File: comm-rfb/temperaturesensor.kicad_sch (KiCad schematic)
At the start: 5 parts, among them U4 MCP9808T-E{slash}MC

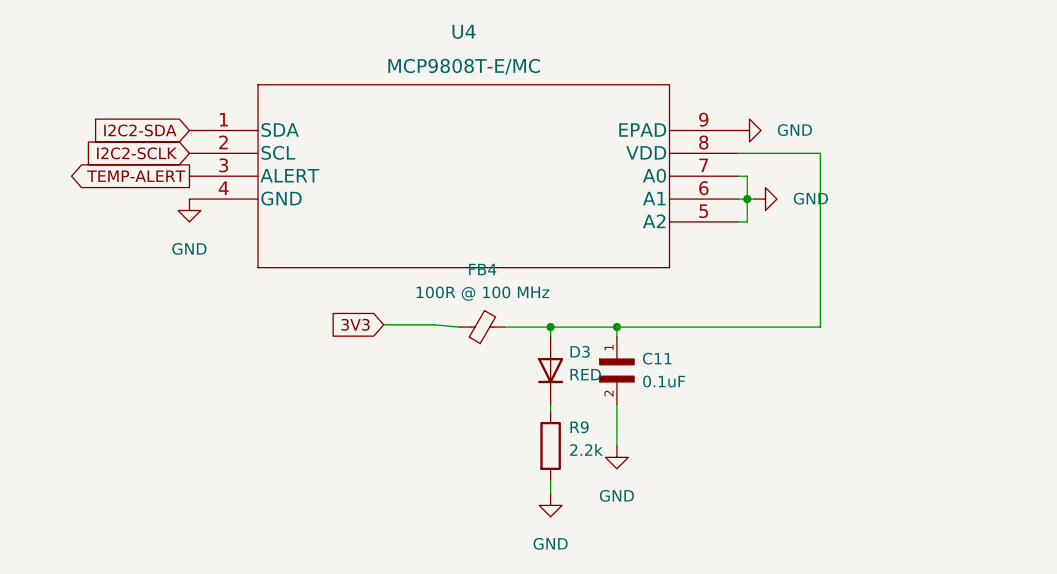
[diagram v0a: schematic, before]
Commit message: comm-rfb: reduce number of sheets in schematic
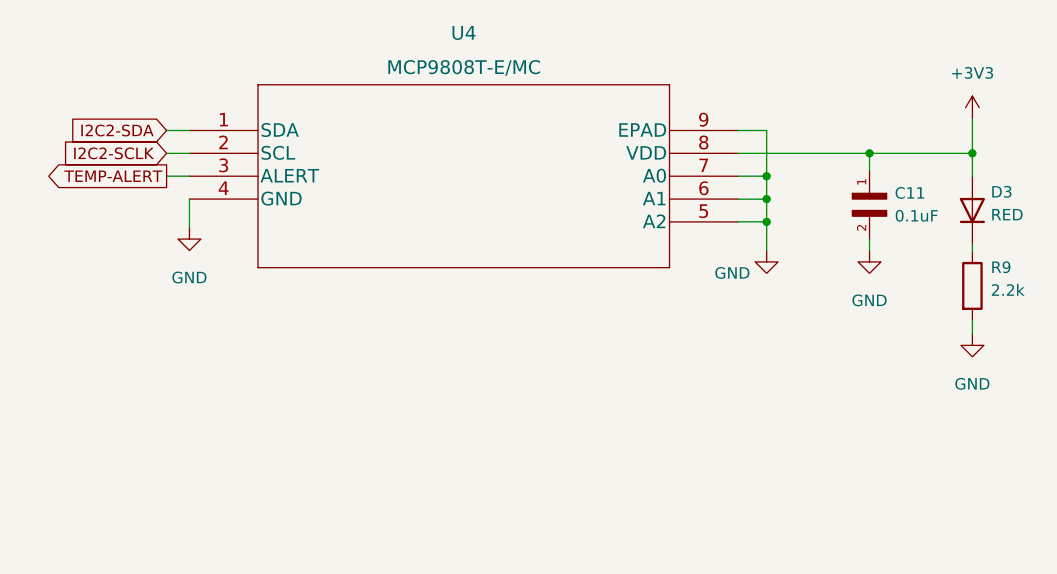
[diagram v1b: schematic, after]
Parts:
- removed FB4: 100R @ 100 MHz, Daughterboard_footprints:BEADC1608X75N, symbol Device:FerriteBead_Small
- removed U4: MCP9808T-E/MC, Daughterboard_footprints:SOP65P490X110-8N, symbol Daughterboard_Symbols:MCP9808T-E{brace}slash}MC
- added U4: MCP9808T-E/MC, qset-footprints:MCP9808T-E&slash_MC, symbol MCP9808T-EMC:MCP9808T-E/MC
- C11: footprint CAPC1608X90N -> Capacitor_SMD:C_0603_1608Metric
- D3: footprint Daughterboard_footprints:CAPC1608X90N -> Diode_SMD:D_0603_1608Metric
- R9: footprint Daughterboard_footprints:RESC1608X55N -> Resistor_SMD:R_0603_1608Metric
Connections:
- net GND: now also U4.4 (GND), U4.5 (A2), U4.6 (A1), U4.7 (A0), U4.9 (EPAD)
- net I2C2-SCLK: now also U4.2 (SCL)
- net I2C2-SDA: now also U4.1 (SDA)
- net TEMP-ALERT: now also U4.3 (ALERT)
- net +3V3: now reaches C11.1, D3.1 (A)
- net +3V3: now also U4.8 (VDD)
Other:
- moved on the sheet: C11, D3, R9
